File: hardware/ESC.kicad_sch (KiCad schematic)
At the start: 85 parts, among them J1 +, J2 -, J3 +, J4 +, J5 +, J6 +, J7 Conn_01x03, J8 +, J9 +, Q1 AGM60P30AP, Q2 AGM60P30AP, Q3 AGM60P30AP, Q4 AGM60P30AP, Q5 AGM60P30AP, Q6 AGM60P30AP, Q7 AGM60P30A, U1 DRV8323RSRGZR, U2 STM32G431CBTx, Y1 X322516MLB4SI

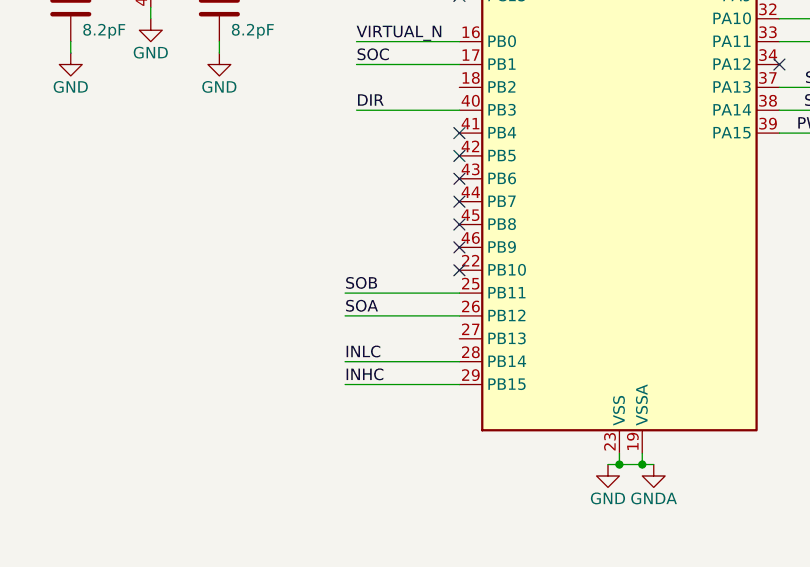
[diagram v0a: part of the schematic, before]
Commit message: finished pcb
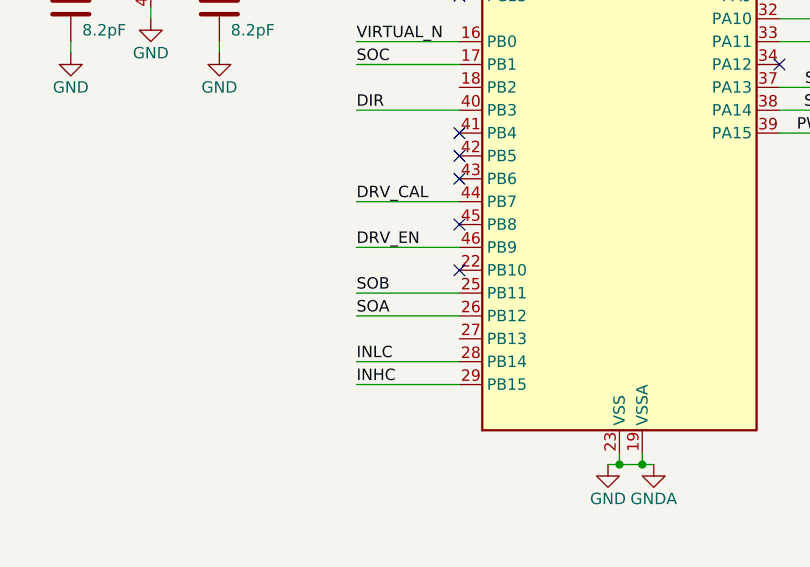
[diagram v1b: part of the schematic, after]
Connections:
- net DRV_CAL: now also U2.44 (PB7)
- net DRV_EN: now also U2.46 (PB9)
- no-connect marks 12 -> 10
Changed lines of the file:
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@@
 	)
 	(no_connect
+		(at 130.81 90.17)
+	)
+	(no_connect
 		(at 130.81 64.77)
 	)
@@
 	)
 	(no_connect
-		(at 130.81 87.63)
-	)
-	(no_connect
-		(at 130.81 90.17)
-	)
-	(no_connect
 		(at 130.81 95.25)
 	)
-	(no_connect
-		(at 130.81 92.71)
-	)
 	(wire
 		(pts
@@
 	(wire
 		(pts
+			(xy 119.38 87.63) (xy 130.81 87.63)
+		)
+		(stroke
+			(width 0)
+			(type default)
+		)
+	)
+	(wire
+		(pts
 			(xy 63.5 53.34) (xy 63.5 54.61)
 		)
@@
 	(wire
 		(pts
+			(xy 119.38 92.71) (xy 130.81 92.71)
+		)
+		(stroke
+			(width 0)
+			(type default)
+		)
+	)
+	(wire
+		(pts
 			(xy 81.28 170.18) (xy 81.28 176.53)
 		)
@@
 	(wire
 		(pts
-			(xy 118.11 107.95) (xy 130.81 107.95)
+			(xy 119.38 107.95) (xy 130.81 107.95)
 		)
 		(stroke
@@
 	(wire
 		(pts
-			(xy 118.11 100.33) (xy 130.81 100.33)
+			(xy 119.38 100.33) (xy 130.81 100.33)
 		)
 		(stroke
@@
 	(wire
 		(pts
-			(xy 118.11 105.41) (xy 130.81 105.41)
+			(xy 119.38 105.41) (xy 130.81 105.41)
 		)
 		(stroke
@@
 	(wire
 		(pts
-			(xy 118.11 97.79) (xy 130.81 97.79)
+			(xy 119.38 97.79) (xy 130.81 97.79)
 		)
 		(stroke
@@
 	)
 	(label "INLC"
-		(at 118.11 105.41 0)
+		(at 119.38 105.41 0)
 		(effects
 			(font
@@
 		)
 	)
+	(label "DRV_EN"
+		(at 119.38 92.71 0)
+		(effects
+			(font
+				(size 1.27 1.27)
+			)
+			(justify left bottom)
+		)
+	)
 	(label "SPB"
 		(at 68.58 176.53 0)
@@
 	)
 	(label "INHC"
-		(at 118.11 107.95 0)
+		(at 119.38 107.95 0)
 		(effects
 			(font
@@
 	)
 	(label "SOB"
-		(at 118.11 97.79 0)
+		(at 119.38 97.79 0)
 		(effects
 			(font
@@
 	)
 	(label "SOA"
-		(at 118.11 100.33 0)
+		(at 119.38 100.33 0)
 		(effects
 			(font
@@
 		(effects
 			(font
+				(size 1.27 1.27)
+			)
+			(justify left bottom)
+		)
+	)
+	(label "DRV_CAL"
+		(at 119.38 87.63 0)
+		(effects
+			(font
